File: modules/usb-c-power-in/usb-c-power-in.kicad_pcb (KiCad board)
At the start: 2 copper layers, 20 x 33 mm, 2 parts, among them J1 Conn_01x02

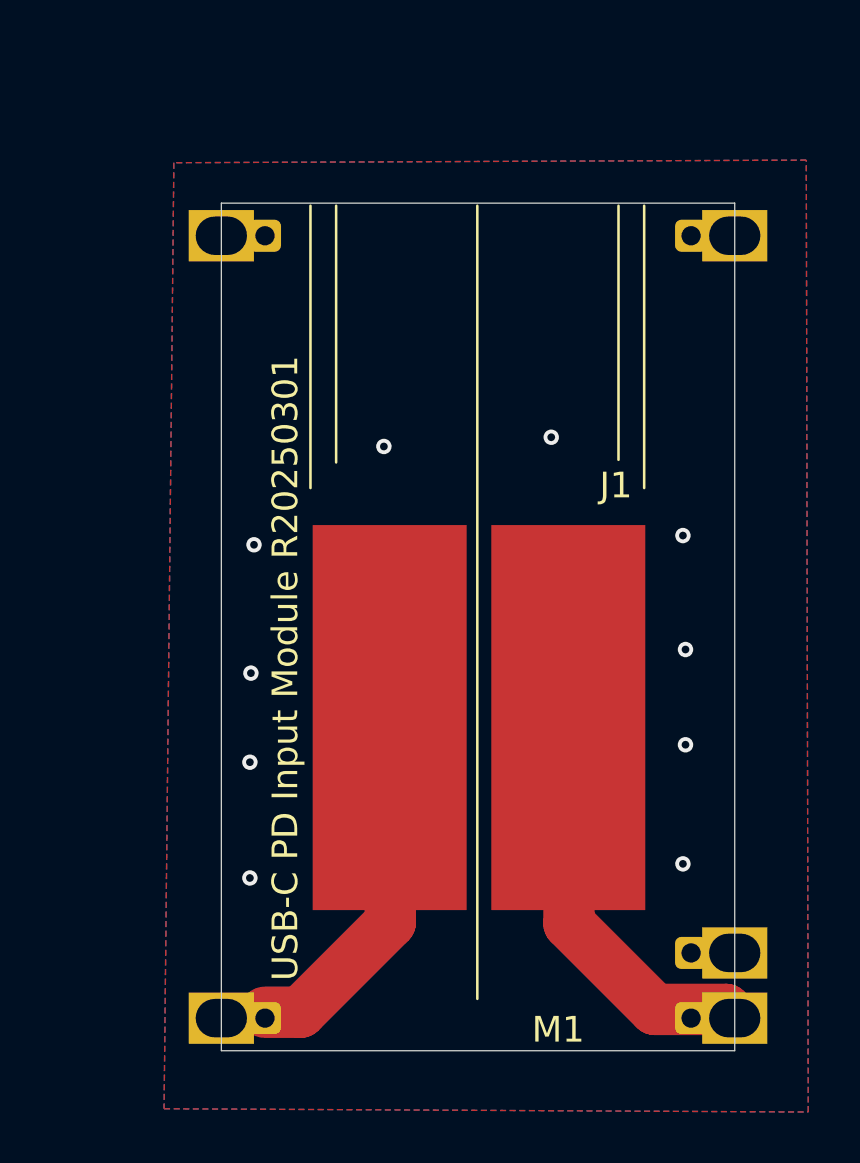
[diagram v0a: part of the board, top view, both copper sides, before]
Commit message: Updating all modules
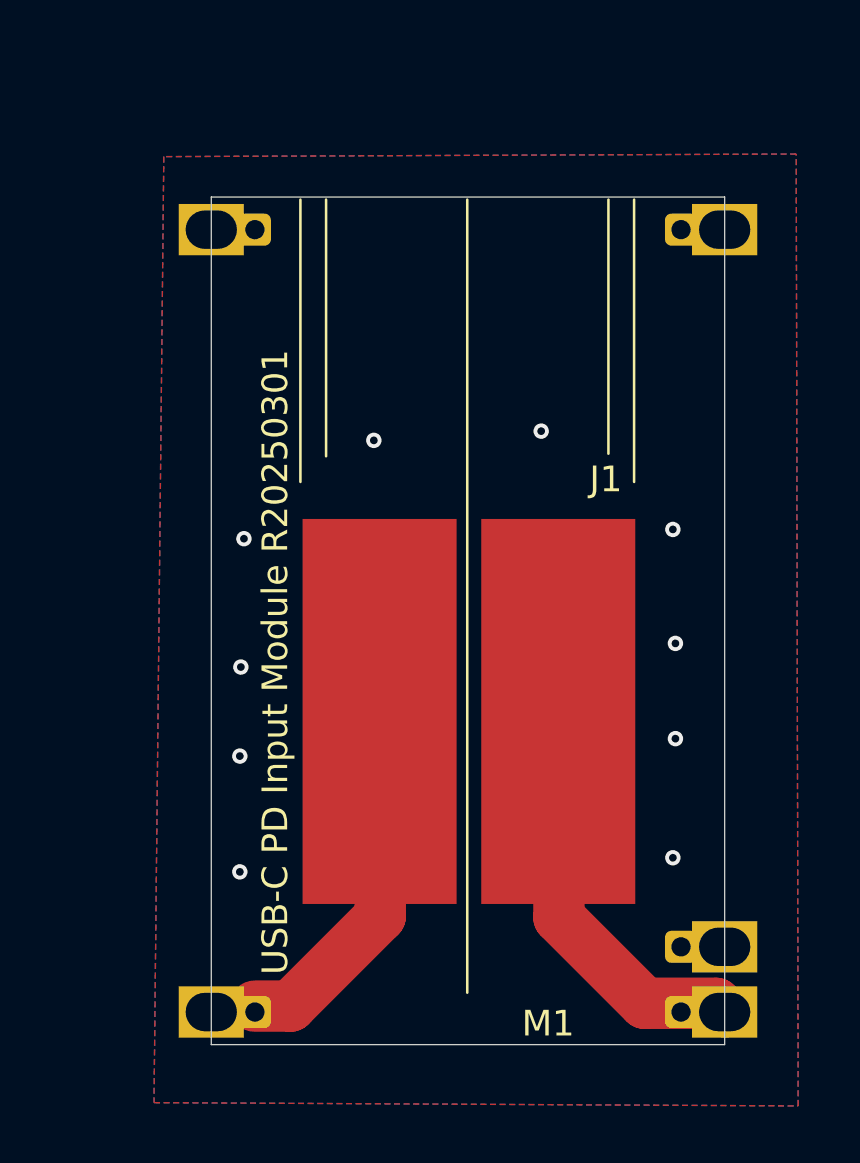
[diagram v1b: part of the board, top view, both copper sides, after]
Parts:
- moved M1 0.46 mm to (49.7, 43.3)
- moved J1 0.46 mm to (50.8, 40.6)
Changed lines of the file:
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@@
 	(footprint "Connector_PinHeader_2.54mm:PinHeader_1x02_P2.54mm_Vertical"
 		(layer "F.Cu")
-		(at 51.181 40.7924 -90)
+		(at 50.789 40.5546 -90)
 		(descr "Through hole straight pin header, 1x02, 2.54mm pitch, single row")
 		(tags "Through hole pin header THT 1x02 2.54mm single row")
@@
 	(footprint "MegaCastle:MegaCastle2x13-Module-I20.0x28.2-M800C00C-SPAREPAD"
 		(layer "F.Cu")
-		(at 50.128 43.5102)
+		(at 49.736 43.2724)
 		(property "Reference" "M1"
 			(at 3.122 15.6898 0)
@@
 			(polygon
 				(pts
-					(xy 40.128 27.0002) (xy 40.128 29.4002) (xy 60.128 29.4002) (xy 60.128 27.0002)
+					(xy 39.736 26.7624) (xy 39.736 29.1624) (xy 59.736 29.1624) (xy 59.736 26.7624)
 				)
 			)
@@
 			(polygon
 				(pts
-					(xy 40.128 60.0202) (xy 40.128 57.6202) (xy 60.128 57.6202) (xy 60.128 60.0202)
+					(xy 39.736 59.7824) (xy 39.736 57.3824) (xy 59.736 57.3824) (xy 59.736 59.7824)
 				)
 			)
@@
 			(polygon
 				(pts
-					(xy 48.143759 28.548792) (xy 48.143759 27.0802) (xy 52.147516 27.0802) (xy 52.147516 28.548792)
+					(xy 47.751759 28.310992) (xy 47.751759 26.8424) (xy 51.755516 26.8424) (xy 51.755516 28.310992)
 				)
 			)
@@
 			(polygon
 				(pts
-					(xy 48.143759 58.471608) (xy 48.143759 59.9402) (xy 52.147516 59.9402) (xy 52.147516 58.471608)
+					(xy 47.751759 58.233808) (xy 47.751759 59.7024) (xy 51.755516 59.7024) (xy 51.755516 58.233808)
 				)
 			)
@@
 	)
 	(gr_line
-		(start 50.1 27.1)
-		(end 50.1 58)
+		(start 49.708 26.8622)
+		(end 49.708 57.7622)
 		(stroke
 			(width 0.1)
@@
 	)
 	(gr_line
-		(start 44.6 27.1)
-		(end 44.6 37.1)
+		(start 44.208 26.8622)
+		(end 44.208 36.8622)
 		(stroke
 			(width 0.1)
@@
 	)
 	(gr_line
-		(start 56.6 27.1)
-		(end 56.6 38.1)
+		(start 56.208 26.8622)
+		(end 56.208 37.8622)
 		(stroke
 			(width 0.1)
@@
 	)
 	(gr_line
-		(start 43.6 27.1)
-		(end 43.6 38.1)
+		(start 43.208 26.8622)
+		(end 43.208 37.8622)
 		(stroke
 			(width 0.1)
@@
 	)
 	(gr_line
-		(start 55.6 27.1)
-		(end 55.6 37)
+		(start 55.208 26.8622)
+		(end 55.208 36.7622)
 		(stroke
 			(width 0.1)
@@
 	)
 	(gr_text "USB-C PD Input Module R20250301"
-		(at 43.2054 57.3024 90)
+		(at 42.8134 57.0646 90)
 		(layer "F.SilkS")
 		(effects
@@
 	)
 	(gr_text "USB-C PD Input Module R20250301\ngithub.com/mega65/\nmegaphone-modular\n"
-		(at 51.689 57.5056 270)
+		(at 51.297 57.2678 270)
 		(layer "B.SilkS")
 		(effects
@@
 	)
 	(segment
-		(start 60.128 58.7502)
-		(end 59.788 58.4102)
+		(start 59.736 58.5124)
+		(end 59.396 58.1724)
 		(width 2)
 		(layer "F.Cu")
@@
 	)
 	(segment
-		(start 57.0132 58.4102)
-		(end 53.6702 55.0672)
+		(start 56.6212 58.1724)
+		(end 53.2782 54.8294)
 		(width 2)
 		(layer "F.Cu")
@@
 	)
 	(segment
-		(start 59.788 58.4102)
-		(end 57.0132 58.4102)
+		(start 59.396 58.1724)
+		(end 56.6212 58.1724)
 		(width 2)
 		(layer "F.Cu")
@@
 	)
 	(segment
-		(start 53.6702 55.0672)
-		(end 53.6702 48.133)
+		(start 53.2782 54.8294)
+		(end 53.2782 47.8952)
 		(width 2)
 		(layer "F.Cu")
@@
 	)
 	(segment
-		(start 46.7106 48.133)
-		(end 46.7106 55.0194)
+		(start 46.3186 47.8952)
+		(end 46.3186 54.7816)
 		(width 2)
 		(layer "F.Cu")
@@
 	)
 	(segment
-		(start 46.7106 55.0194)
-		(end 43.2098 58.5202)
+		(start 46.3186 54.7816)
+		(end 42.8178 58.2824)
 		(width 2)
 		(layer "F.Cu")
@@
 	)
 	(segment
-		(start 43.2098 58.5202)
-		(end 41.828 58.5202)
+		(start 42.8178 58.2824)
+		(end 41.436 58.2824)
 		(width 2)
 		(layer "F.Cu")
@@
 	)
 	(via
-		(at 52.98 36.12)
-		(size 0.6)
-		(drill 0.3)
-		(layers "F.Cu" "B.Cu")
-		(free yes)
-		(net 5)
-	)
-	(via
-		(at 46.46 36.48)
-		(size 0.6)
-		(drill 0.3)
-		(layers "F.Cu" "B.Cu")
-		(free yes)
-		(net 5)
-	)
-	(via
-		(at 41.24 48.78)
-		(size 0.6)
-		(drill 0.3)
-		(layers "F.Cu" "B.Cu")
-		(free yes)
-		(net 5)
-	)
-	(via
-		(at 58.11 39.95)
-		(size 0.6)
-		(drill 0.3)
-		(layers "F.Cu" "B.Cu")
-		(free yes)
-		(net 5)
-	)
-	(via
-		(at 41.4 40.31)
-		(size 0.6)
-		(drill 0.3)
-		(layers "F.Cu" "B.Cu")
-		(free yes)
-		(net 5)
-	)
-	(via
-		(at 58.21 44.39)
-		(size 0.6)
-		(drill 0.3)
-		(layers "F.Cu" "B.Cu")
-		(free yes)
-		(net 5)
-	)
-	(via
-		(at 41.24 53.29)
-		(size 0.6)
-		(drill 0.3)
-		(layers "F.Cu" "B.Cu")
-		(free yes)
-		(net 5)
-	)
-	(via
-		(at 58.21 48.1)
-		(size 0.6)
-		(drill 0.3)
-		(layers "F.Cu" "B.Cu")
-		(free yes)
-		(net 5)
-	)
-	(via
-		(at 58.11 52.74)
-		(size 0.6)
-		(drill 0.3)
-		(layers "F.Cu" "B.Cu")
-		(free yes)
-		(net 5)
-	)
-	(via
-		(at 41.28 45.31)
+		(at 52.588 35.8822)
+		(size 0.6)
+		(drill 0.3)
+		(layers "F.Cu" "B.Cu")
+		(free yes)
+		(net 5)
+	)
+	(via
+		(at 46.068 36.2422)
+		(size 0.6)
+		(drill 0.3)
+		(layers "F.Cu" "B.Cu")
+		(free yes)
+		(net 5)
+	)
+	(via
+		(at 40.848 48.5422)
+		(size 0.6)
+		(drill 0.3)
+		(layers "F.Cu" "B.Cu")
+		(free yes)
+		(net 5)
+	)
+	(via
+		(at 57.718 39.7122)
+		(size 0.6)
+		(drill 0.3)
+		(layers "F.Cu" "B.Cu")
+		(free yes)
+		(net 5)
+	)
+	(via
+		(at 41.008 40.0722)
+		(size 0.6)
+		(drill 0.3)
+		(layers "F.Cu" "B.Cu")
+		(free yes)
+		(net 5)
+	)
+	(via
+		(at 57.818 44.1522)
+		(size 0.6)
+		(drill 0.3)
+		(layers "F.Cu" "B.Cu")
+		(free yes)
+		(net 5)
+	)
+	(via
+		(at 40.848 53.0522)
+		(size 0.6)
+		(drill 0.3)
+		(layers "F.Cu" "B.Cu")
+		(free yes)
+		(net 5)
+	)
+	(via
+		(at 57.818 47.8622)
+		(size 0.6)
+		(drill 0.3)
+		(layers "F.Cu" "B.Cu")
+		(free yes)
+		(net 5)
+	)
+	(via
+		(at 57.718 52.5022)
+		(size 0.6)
+		(drill 0.3)
+		(layers "F.Cu" "B.Cu")
+		(free yes)
+		(net 5)
+	)
+	(via
+		(at 40.888 45.0722)
 		(size 0.6)
 		(drill 0.3)
@@
 		(polygon
 			(pts
-				(xy 38.2778 25.4254) (xy 37.8968 62.2808) (xy 62.992 62.4078) (xy 62.9158 25.3238)
-			)
-		)
+				(xy 37.8858 25.1876) (xy 37.5048 62.043) (xy 62.6 62.17) (xy 62.5238 25.086)
+			)
+		)
